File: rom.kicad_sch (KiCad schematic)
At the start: 3 parts, among them IC17 27C256, IC18 74LS08

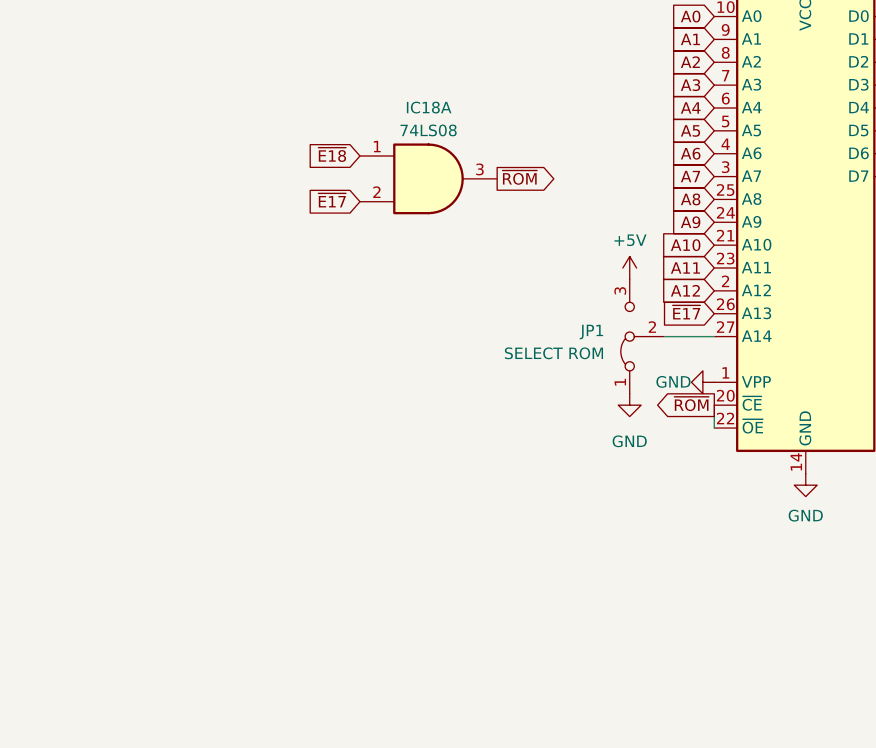
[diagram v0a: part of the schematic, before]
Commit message: handle 27C512
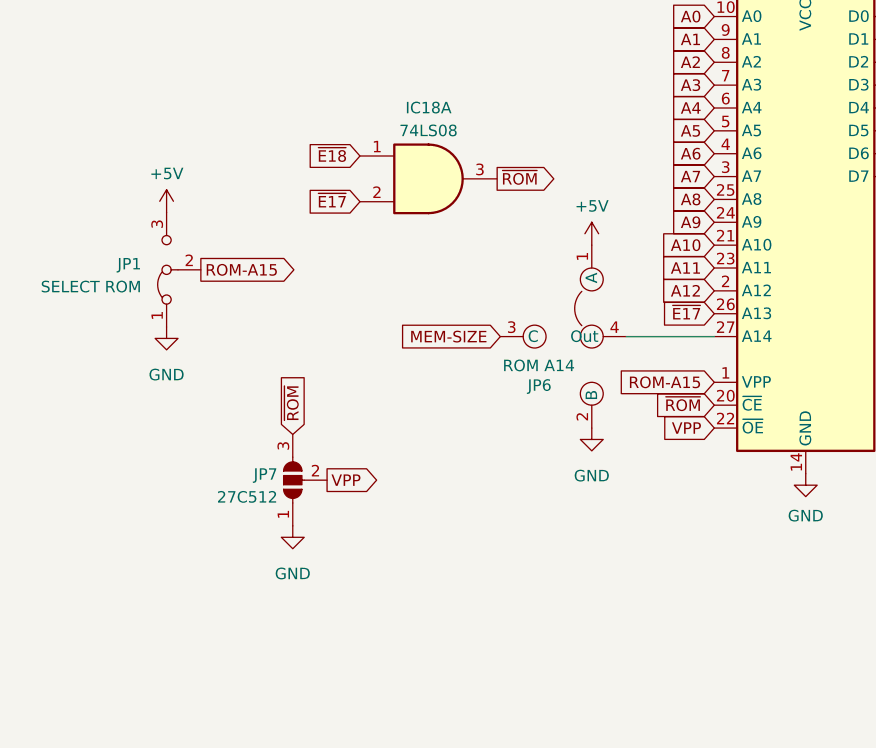
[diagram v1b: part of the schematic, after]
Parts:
- added JP6: ROM A14, Dragon:Jumper_4, symbol vdg:Jumper_4
- added JP7: 27C512, Jumper:SolderJumper-3_P1.3mm_Open_Pad1.0x1.5mm, symbol Jumper:SolderJumper_3_Open
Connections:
- net +5V: now also JP6.1 (A)
- net GND: now also JP6.2 (B), JP7.1 (A); no longer IC17.1 (VPP)
- net ~{ROM}: now also JP7.3 (B); no longer IC17.22 (~{OE})
- net at IC17.27 (A14): now also JP6.4 (Out); no longer JP1.2 (C)
- new net MEM-SIZE: JP6.3 (C)
- new net ROM-A15: IC17.1 (VPP), JP1.2 (C)
- new net VPP: IC17.22 (~{OE}), JP7.2 (C)
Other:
- moved on the sheet: JP1
